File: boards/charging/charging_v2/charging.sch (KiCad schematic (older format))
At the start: 56 parts, among them IC1 ATMEGA16M1, J1 CONN_02X03, J2 Ampseal_8, J3 Ultrafit_4, J4 Ultrafit_4, J5 micromatch_female_TOP_ENTRY_l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, P1 CONN_02X03, U1 CAN_Transceiver, U2 TPS561201, U3 CAN_Transceiver, U4 RJ45_RA, U5 ATMEGA328P-AU, Y1 Crystal_SMD, Y2 Crystal_SMD

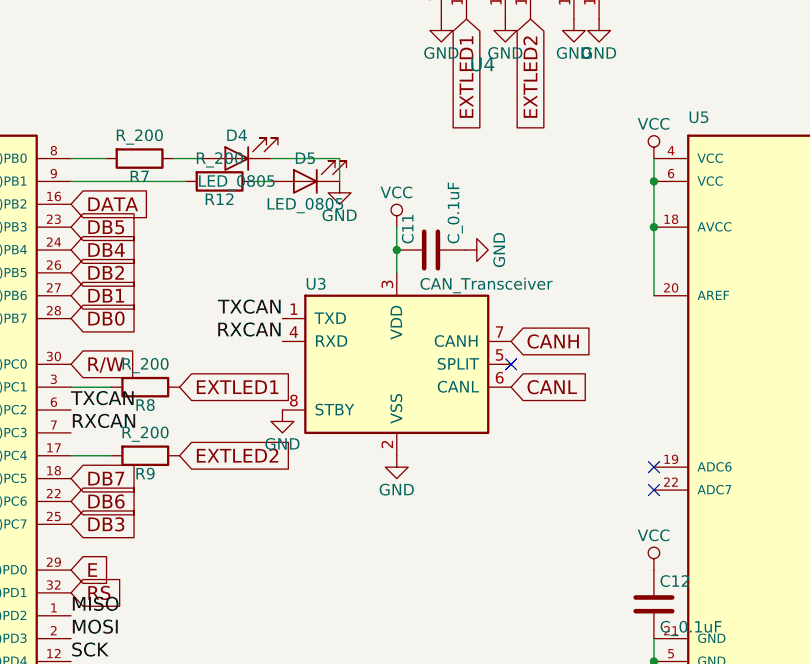
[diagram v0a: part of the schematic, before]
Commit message: charging v2
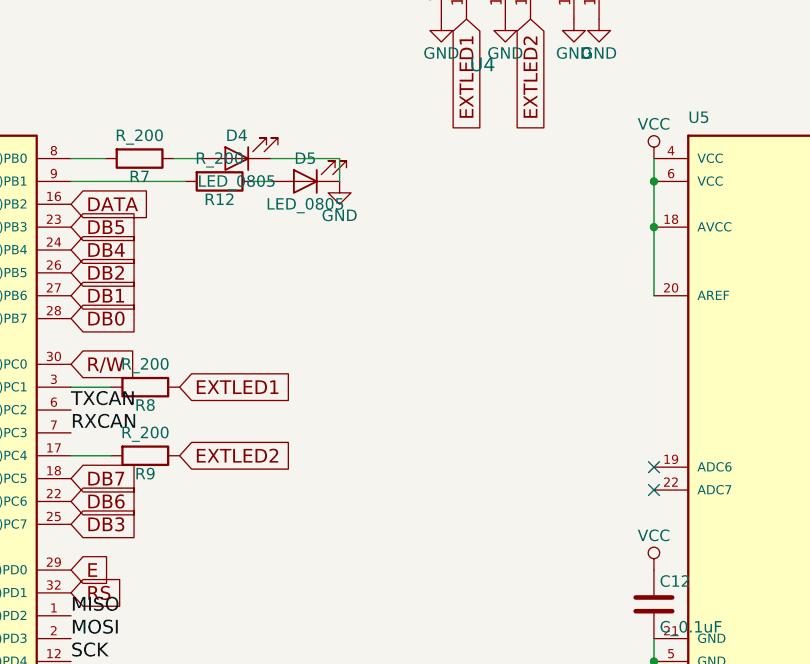
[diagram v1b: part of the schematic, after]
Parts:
- removed C11: C_0.1uF, footprints:C_0805_OEM, symbol C_0.1uF
- removed U3: CAN_Transceiver, footprints:SOIC-8_3.9x4.9mm_Pitch1.27mm_OEM, symbol CAN_Transceiver
- J2: footprint (none) -> footprints:Ampseal_8; MPN (none) -> MRJ-5381-01-ND; PurchasingLink (none) -> https://www.digikey.com/product-detail/en/amphenol-commerci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
- RV1: footprint (none) -> footprints:Potentiometer_Trimmer_Bourns_TCC3
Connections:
- no-connect marks 18 -> 17
